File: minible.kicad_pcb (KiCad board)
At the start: 2 copper layers, 8.9 x 8.9 mm, 28 parts, among them U2 nRF52833_QDxx, Y2 Crystal_GND24

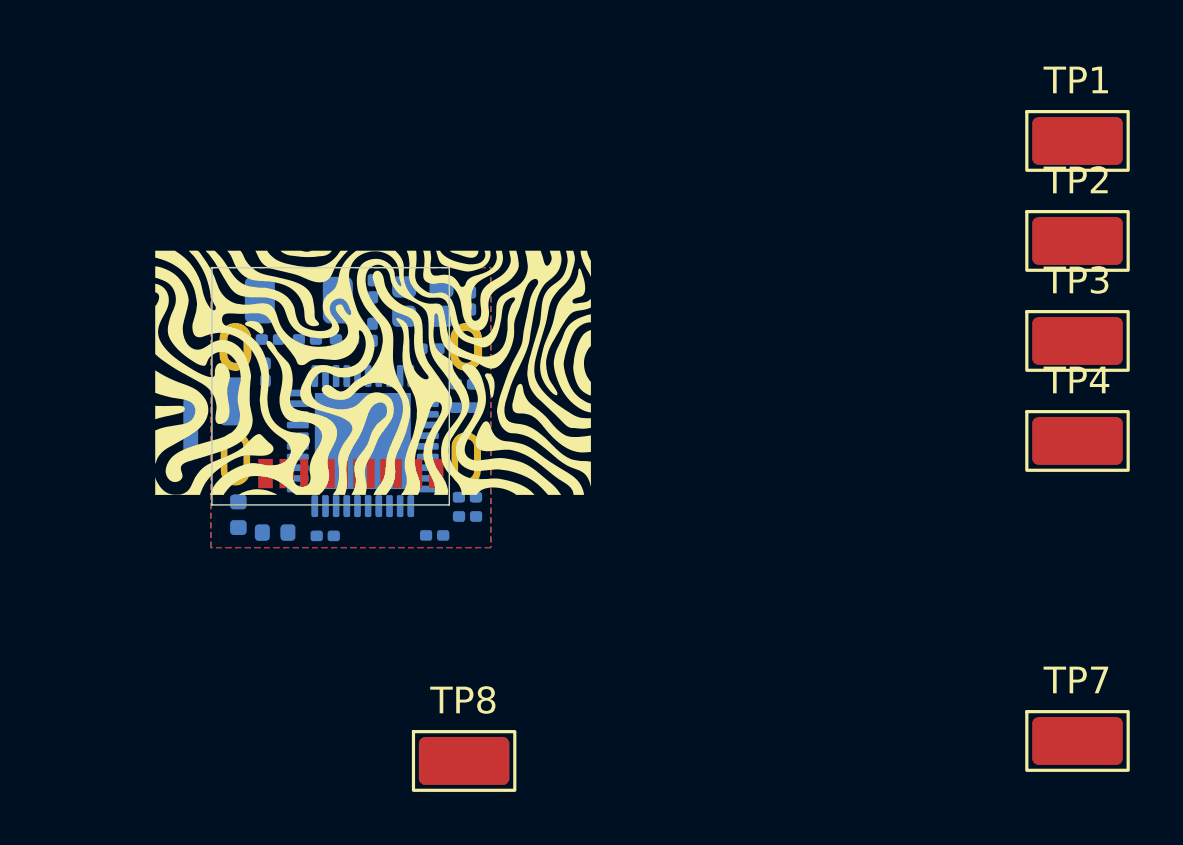
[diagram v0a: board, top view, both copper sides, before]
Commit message: finish PCB
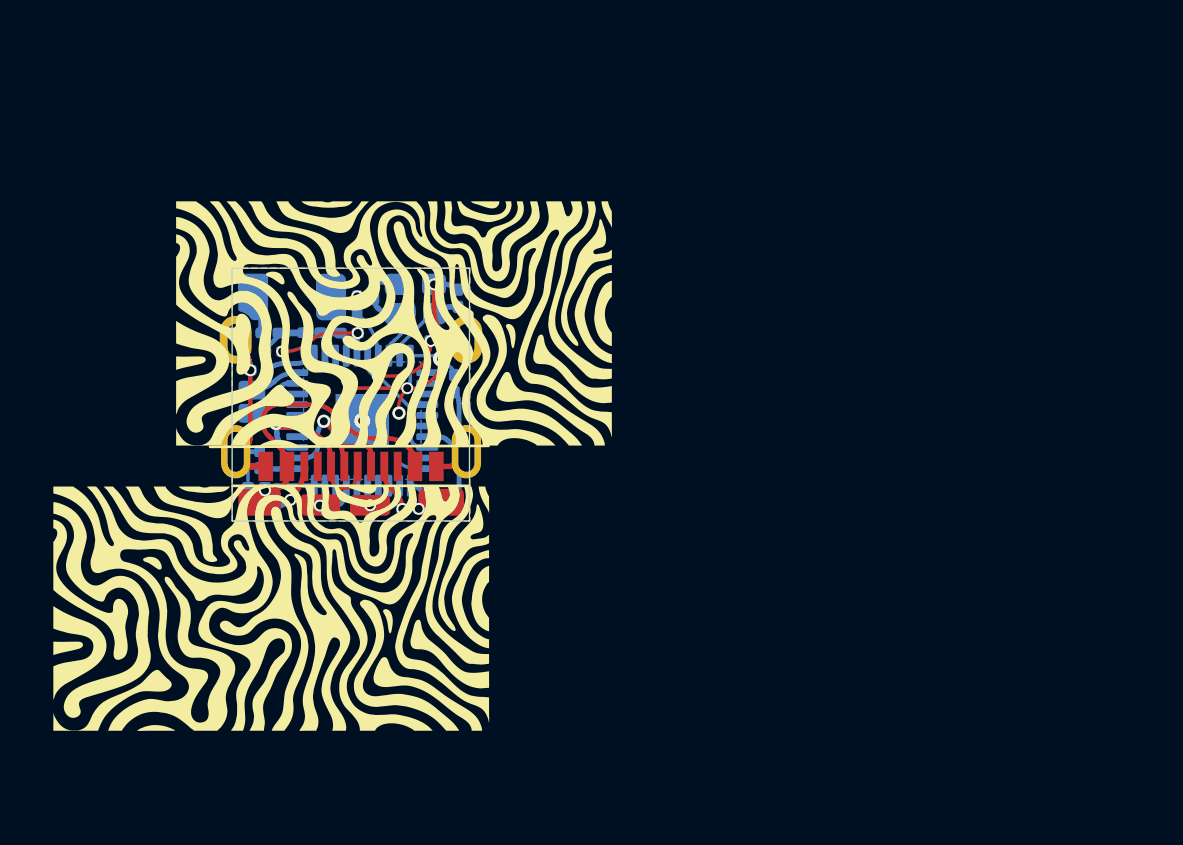
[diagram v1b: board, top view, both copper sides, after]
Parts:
- removed C6: 100nF, Capacitor_SMD:C_0201_0603Metric
- removed TP1, TP3: TestPoint, TestPoint:TestPoint_Keystone_5015_Micro_Mini
- C5, C8: value 4.7uF -> 1uF; footprint Capacitor_SMD:C_0402_1005Metric -> Capacitor_SMD:C_0201_0603Metric
- moved TP4 28.5 mm to (163.1, 94.9), turned to 180 degrees
- moved TP2 28.3 mm to (165.0, 94.9)
- moved TP7 25.5 mm to (167.6, 94.8)
- moved TP8 12.4 mm to (160.8, 94.8)
- moved C11 5.97 mm to (167.6, 88.7)
- moved C15 3.78 mm to (161.4, 89.1), turned to 180 degrees
- moved C10 3.19 mm to (164.5, 87.4), turned to 90 degrees
- moved C14 2.97 mm to (164.2, 88.5), turned to 180 degrees
- moved R1 2.82 mm to (160.7, 94.9), turned to 0 degrees
- moved L2 2.80 mm to (161.2, 88.5), turned to 180 degrees
- moved TP6 2.35 mm to (160.5, 91.5)
- moved C8 2.22 mm to (160.8, 93.2), turned to 90 degrees
- moved C5 1.83 mm to (160.7, 94.2)
- moved R2 1.34 mm to (166.5, 95.0)
- moved C3 0.98 mm to (168.1, 90.3), turned to -90 degrees
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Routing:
- net GND: track 1.59 -> 21.8 mm, vias 0 -> 6
- net VBUS: track 0.00 -> 13.5 mm, vias 0 -> 1
- net VDD: track 0.00 -> 9.70 mm, vias 0 -> 4
- net /DEC4_6: track 0.00 -> 7.38 mm, vias 0 -> 2
- net /D+: track 0.00 -> 6.66 mm, vias 0 -> 1
- net /D-: track 0.00 -> 6.17 mm, vias 0 -> 1
- net /XC1: track 0.00 -> 4.15 mm
- net /VSS_PA: track 0.00 -> 3.94 mm, vias 0 -> 2
- net /XC2: track 0.00 -> 3.10 mm
- net Net-(USB1-CC2): track 0.00 -> 2.62 mm, vias 0 -> 1
- net /SWDIO: track 0.00 -> 2.27 mm
- net /SWDCLK: track 0.00 -> 1.97 mm
- net Net-(USB1-CC1): track 0.00 -> 1.90 mm, vias 0 -> 1
- net /DEC5: track 0.00 -> 1.89 mm
- net Net-(C15-Pad2): track 0.00 -> 1.82 mm
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- added copper zone on B.Cu, net VDD
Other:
- board size 8.9 x 8.9 mm -> 8.9 x 9.5 mm
- board text added: "ble"
- board text added: "mi"
- board text added: "ni"
- board text added: "v0.1"
